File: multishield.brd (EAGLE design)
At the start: 57.6 x 53.7 mm, 20 parts, among them CN1 3P-2.54-90D, J2 2x16p-2.54, J4 2x6p-2.54, K2 TS-1101F, M1 ARDUINO_R3_ICSP, SW1 SK-12D01, U1 AD595AQ-DIP14, U2 ATMEGA328P_PDIP, Y1 16MHZ

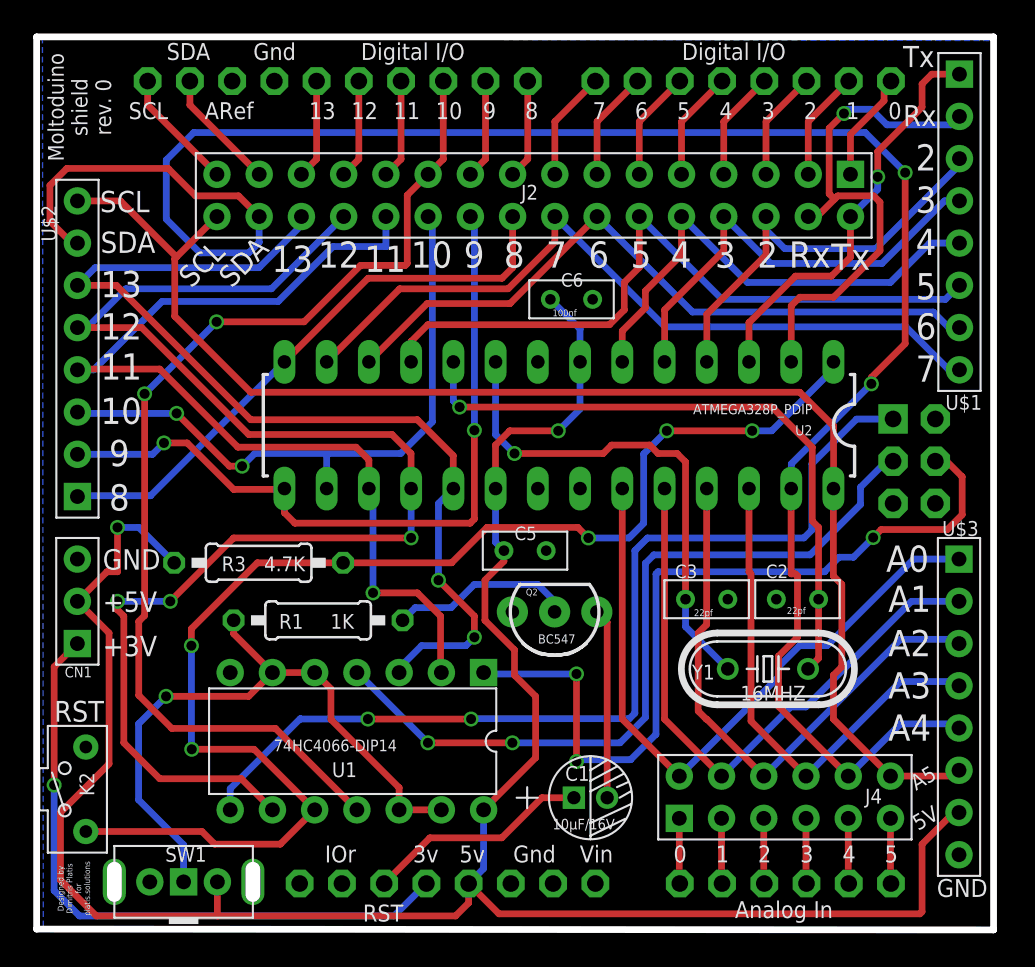
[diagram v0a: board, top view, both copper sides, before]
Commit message: rev 1
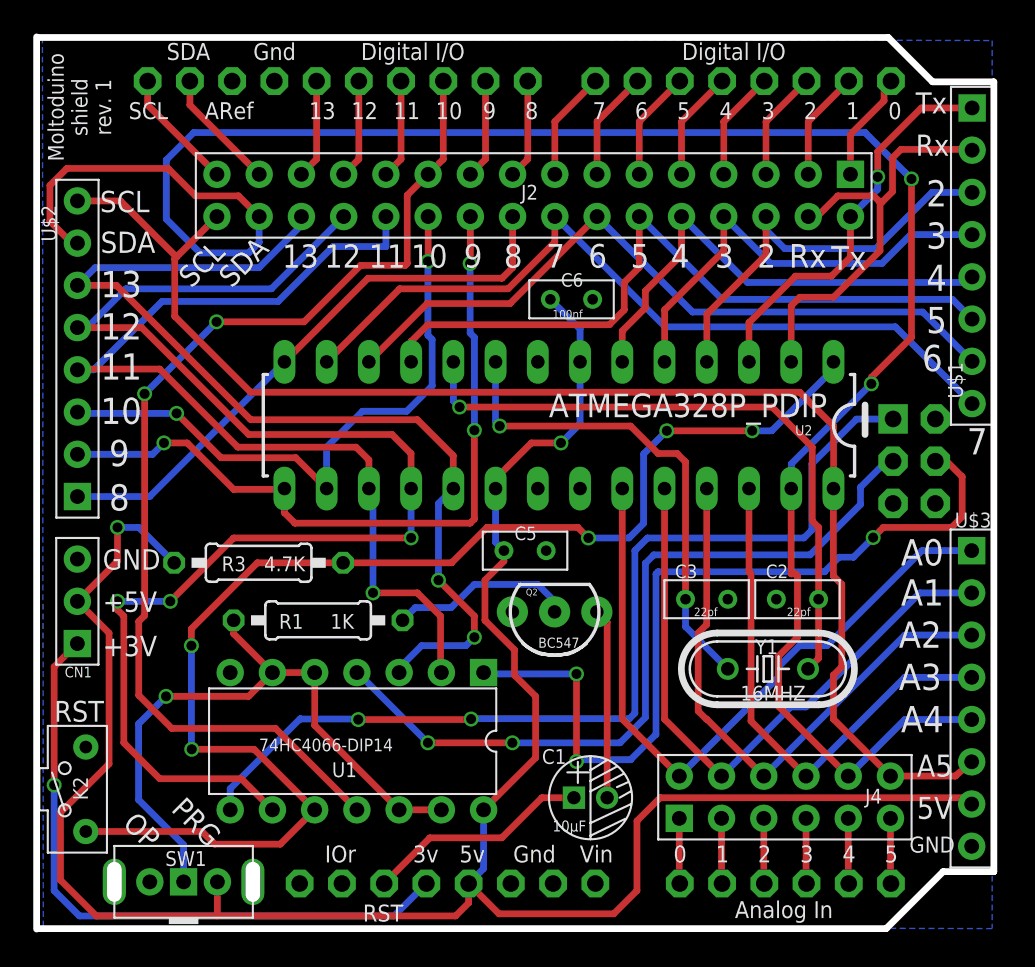
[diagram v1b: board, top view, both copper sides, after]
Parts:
- added U$4: (no value), adafruit:OSHWLOGO_BACK_0.2
- C1: value 10µF/16V -> 10µF
- moved U$1 2.17 mm to (59.0, 40.6)
- moved U$3 0.92 mm to (59.0, 14.0)
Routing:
- net N$26: track 31.3 -> 26.1 mm, vias 1 -> 0
- net N$41: track 41.9 -> 43.5 mm
- net N$32: track 46.4 -> 48.0 mm
- net N$49: track 126.2 -> 127.3 mm
- net N$46: track 37.3 -> 38.3 mm
- net N$45: track 41.3 -> 42.3 mm
- net N$50: track 83.9 -> 84.9 mm
- net N$30: track 42.5 -> 43.4 mm
- net N$25: track 24.8 -> 23.9 mm
- net N$57: track 30.4 -> 29.5 mm
- net N$35: track 38.4 -> 37.6 mm
- net N$48: track 30.4 -> 31.1 mm
- net N$47: track 34.4 -> 35.2 mm
- net N$34: track 45.4 -> 45.5 mm, vias 2 -> 3
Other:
- outline, holes or cut-outs redrawn
- board text added: "Moltoduino shield rev. 1"
- board text added: "OP"
- board text added: "PRG"
- board text removed: "Designed by Dimitris Platis for platis.solutions"
- board text removed: "Moltoduino shield rev. 0"
